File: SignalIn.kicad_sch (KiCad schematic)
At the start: 38 parts, among them J2 AC3FAH2-XLR, U4 AD8512, U6 AD8512, U7 AD8512

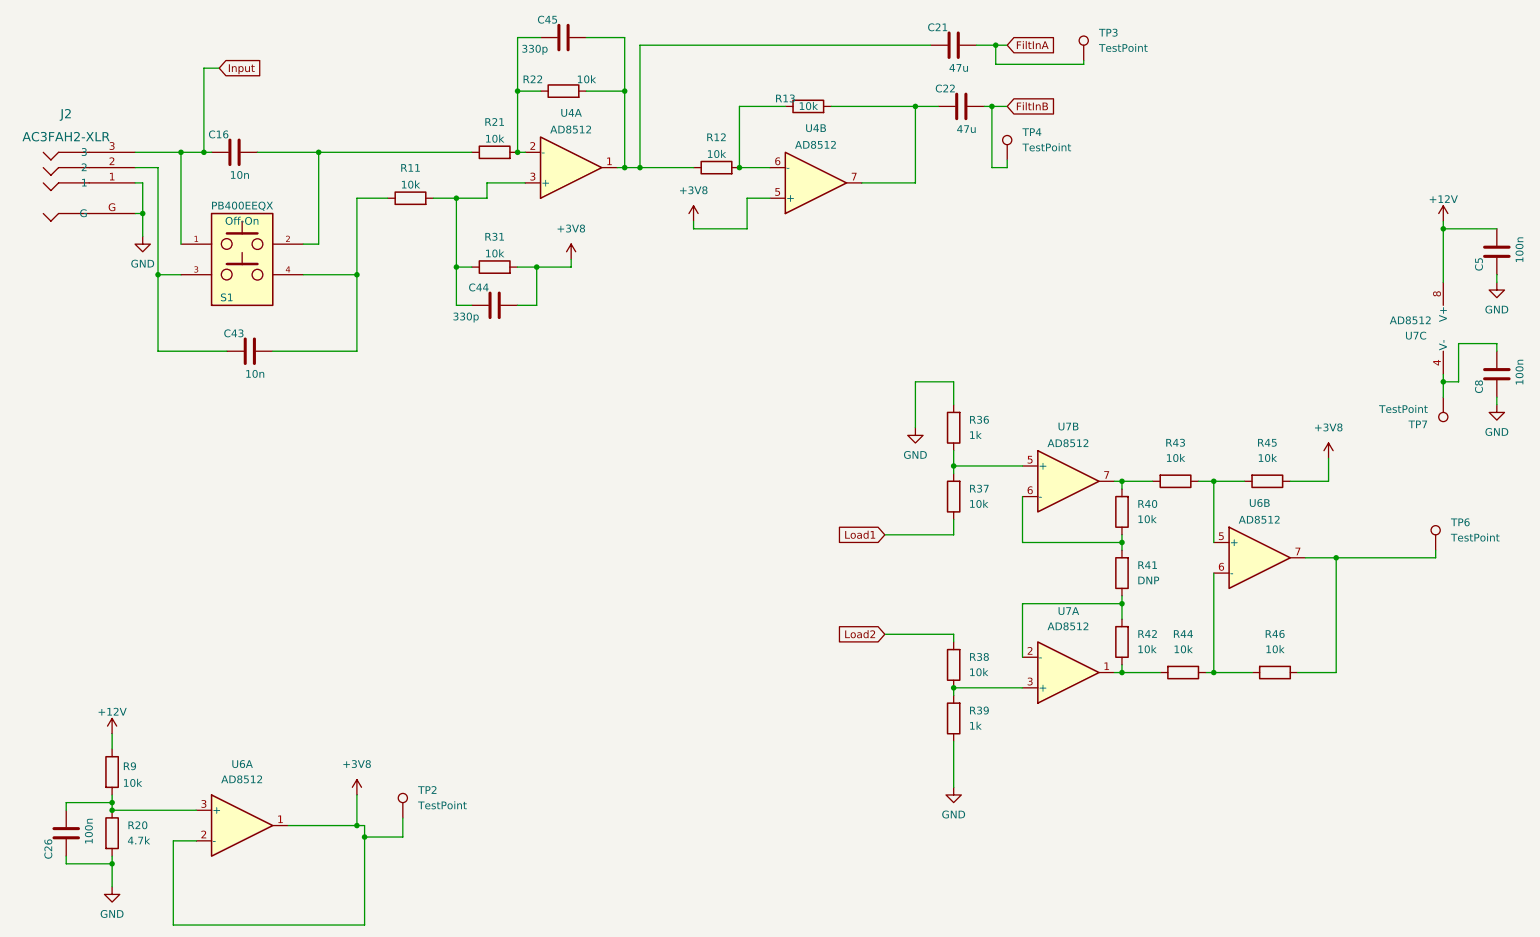
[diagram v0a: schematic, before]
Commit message: Pre mfg, Rev B
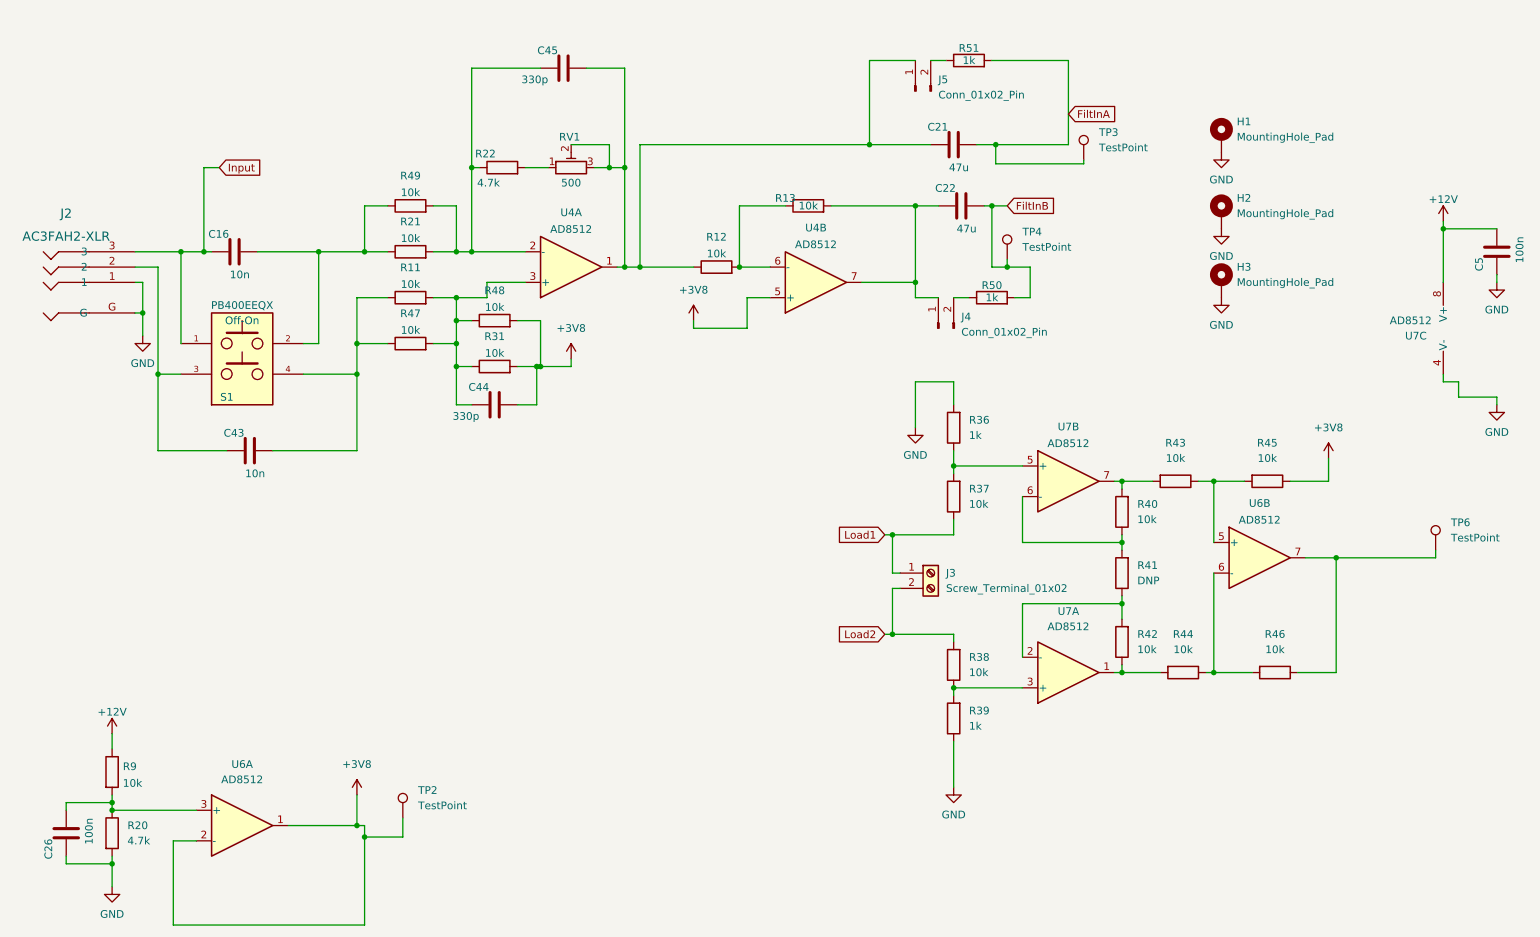
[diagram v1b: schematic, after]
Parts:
- removed C8: 100n, Capacitor_SMD:C_0805_2012Metric, symbol Device:C
- removed TP7: TestPoint, TestPoint:TestPoint_THTPad_1.0x1.0mm_Drill0.5mm, symbol Connector:TestPoint
- added H1, H2, H3: MountingHole_Pad, MountingHole:MountingHole_3.2mm_M3_Pad_Via, symbol Mechanical:MountingHole_Pad
- added J3: Screw_Terminal_01x02, TerminalBlock_Phoenix:TerminalBlock_Phoenix_MKDS-1,5-2-5.08_1x02_P5.08mm_Horizontal, symbol Connector:Screw_Terminal_01x02
- added J4, J5: Conn_01x02_Pin, Connector_PinHeader_1.27mm:PinHeader_1x02_P1.27mm_Vertical, symbol Connector:Conn_01x02_Pin
- added R47, R48, R49: 10k, Resistor_SMD:R_0805_2012Metric, symbol Device:R
- added R50, R51: 1k, Resistor_SMD:R_0805_2012Metric, symbol Device:R
- added RV1: 500, Potentiometer_THT:Potentiometer_Bourns_3296W_Vertical, symbol Device:R_Potentiometer_Trim
- R22: value 10k -> 4.7k
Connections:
- net +3V8: now also R48.2
- net FiltInA: now also R51.2
- net FiltInB: now also R50.2
- net GND: now also U7.4 (V-), H1.1, H2.1, H3.1
- net Load1: now also J3.1 (Pin_1)
- net Load2: now also J3.2 (Pin_2)
- net at C44.1, R11.2, R31.1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: now also R47.2, R48.1
- net at C22.1, R13.2, U4.7: now also J4.1 (Pin_1)
- net at C45.1, R21.2, R22.1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: now also R49.2
- net at C21.1, C45.2, R12.1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: now also J5.1 (Pin_1), RV1.2, RV1.3; no longer R22.2
- net at C16.2, R21.1, S1.2: now also R49.1
- net at C43.2, R11.1, S1.4: now also R47.1
- new net: R22.2, RV1.1
- new net: J4.2 (Pin_2), R50.1
- new net: J5.2 (Pin_2), R51.1
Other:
- moved on the sheet: C16, C21, C22, C43, C44, C45, J2, R11, R12, R13, R21, R22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
